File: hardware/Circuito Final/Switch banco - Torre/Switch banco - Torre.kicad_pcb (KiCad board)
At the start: 2 copper layers, 98.6 x 48.6 mm, 69 parts, among them J1 Conn_01x07, J2 Conn_02x07_Odd_Even, J3 Conn_01x07, Q1 MMBFJ112, Q1_1 MMBT2222A, Q3 MMBT2222A, U1 74HC595, U2 74HC4051

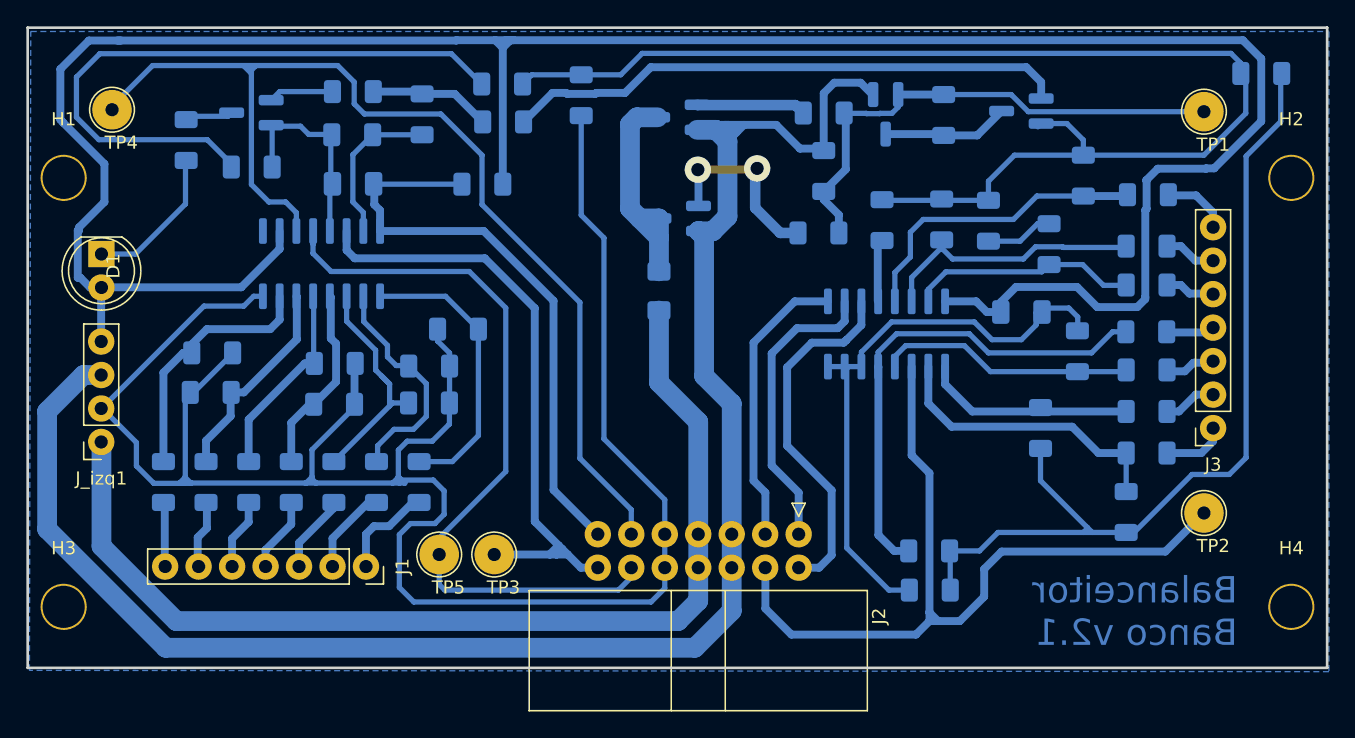
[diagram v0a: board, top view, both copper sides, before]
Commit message: prueba del mux, y bitacora del dia
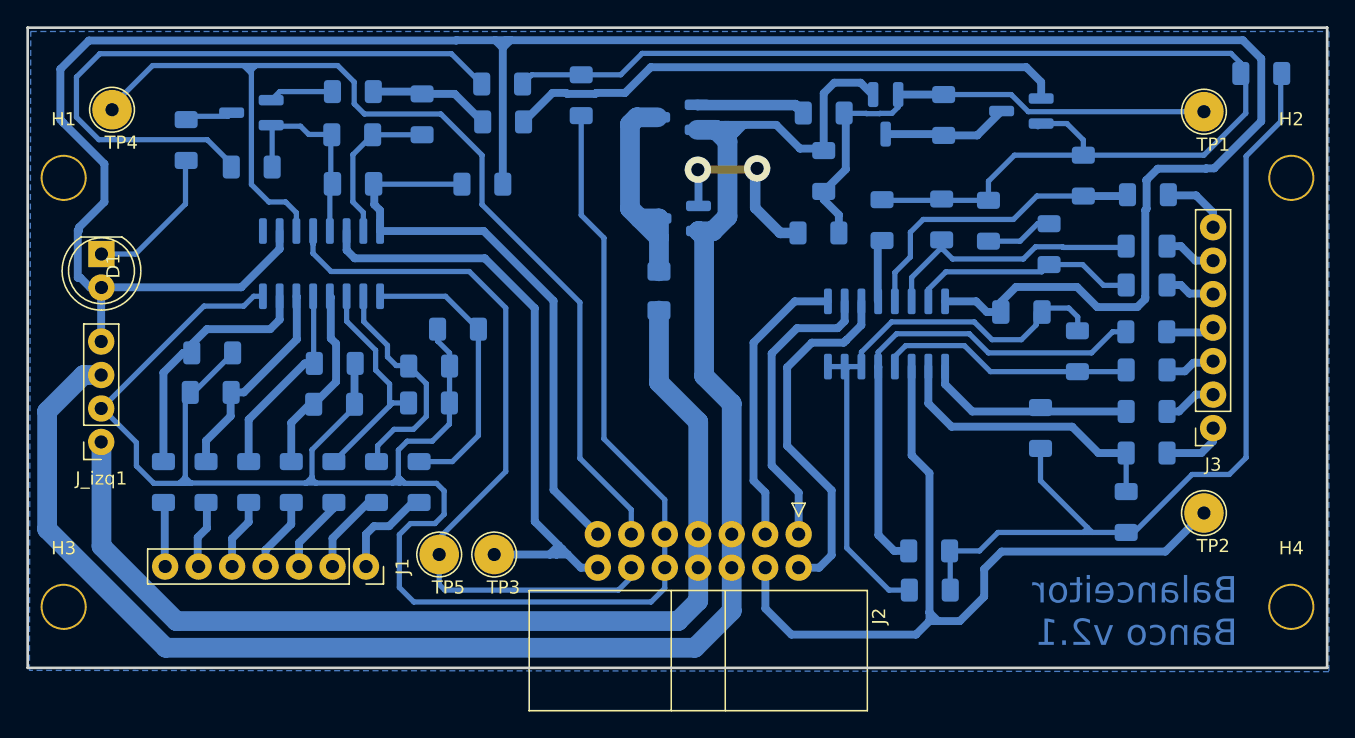
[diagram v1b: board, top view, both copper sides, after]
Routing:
- net GND: track 433.7 -> 428.3 mm
- net /latch: track 57.0 -> 55.0 mm
- net Net-(U2-A7): track 20.0 -> 18.6 mm
- net Net-(U1-QD): track 18.5 -> 17.2 mm
- net /cell_neg4: track 4.02 -> 2.87 mm
- net /Vcc: track 233.7 -> 232.8 mm
- net Net-(U1-QC): track 17.9 -> 17.1 mm
- net /clock: track 83.5 -> 82.7 mm
- net /DATA: track 47.8 -> 47.1 mm
- net Net-(Q1-S): track 39.5 -> 38.9 mm
- net /salida_adc: track 62.9 -> 62.3 mm
- net Net-(U2-A1): track 21.2 -> 20.7 mm
- net Net-(U2-A3): track 4.76 -> 4.26 mm
